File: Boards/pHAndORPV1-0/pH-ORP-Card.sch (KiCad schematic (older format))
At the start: 118 parts, among them IC1 PIC32MM0064GPM028, P1 ICSP, P2 AquaPicBus, P3 Power, P4 pH, P5 pH/ORP, Q1 NX7002AK, Q2 NX7002AK, Q3 NX7002AK, Q4 AO3407A, Q5 MMBT3904, Q6 MMBT3904, Q7 AO3407A, Q8 AO3407A, U1 AP2114H, U10 LTC2483, U11 Si8602, U12 TC7660, U2 ST485EC, U3 LMC6061, U4 TLV272, U5 LTC2483, U6 Si8602, U7 TC7660, U8 LMC6061, U9 TLV272, X1 8MHz

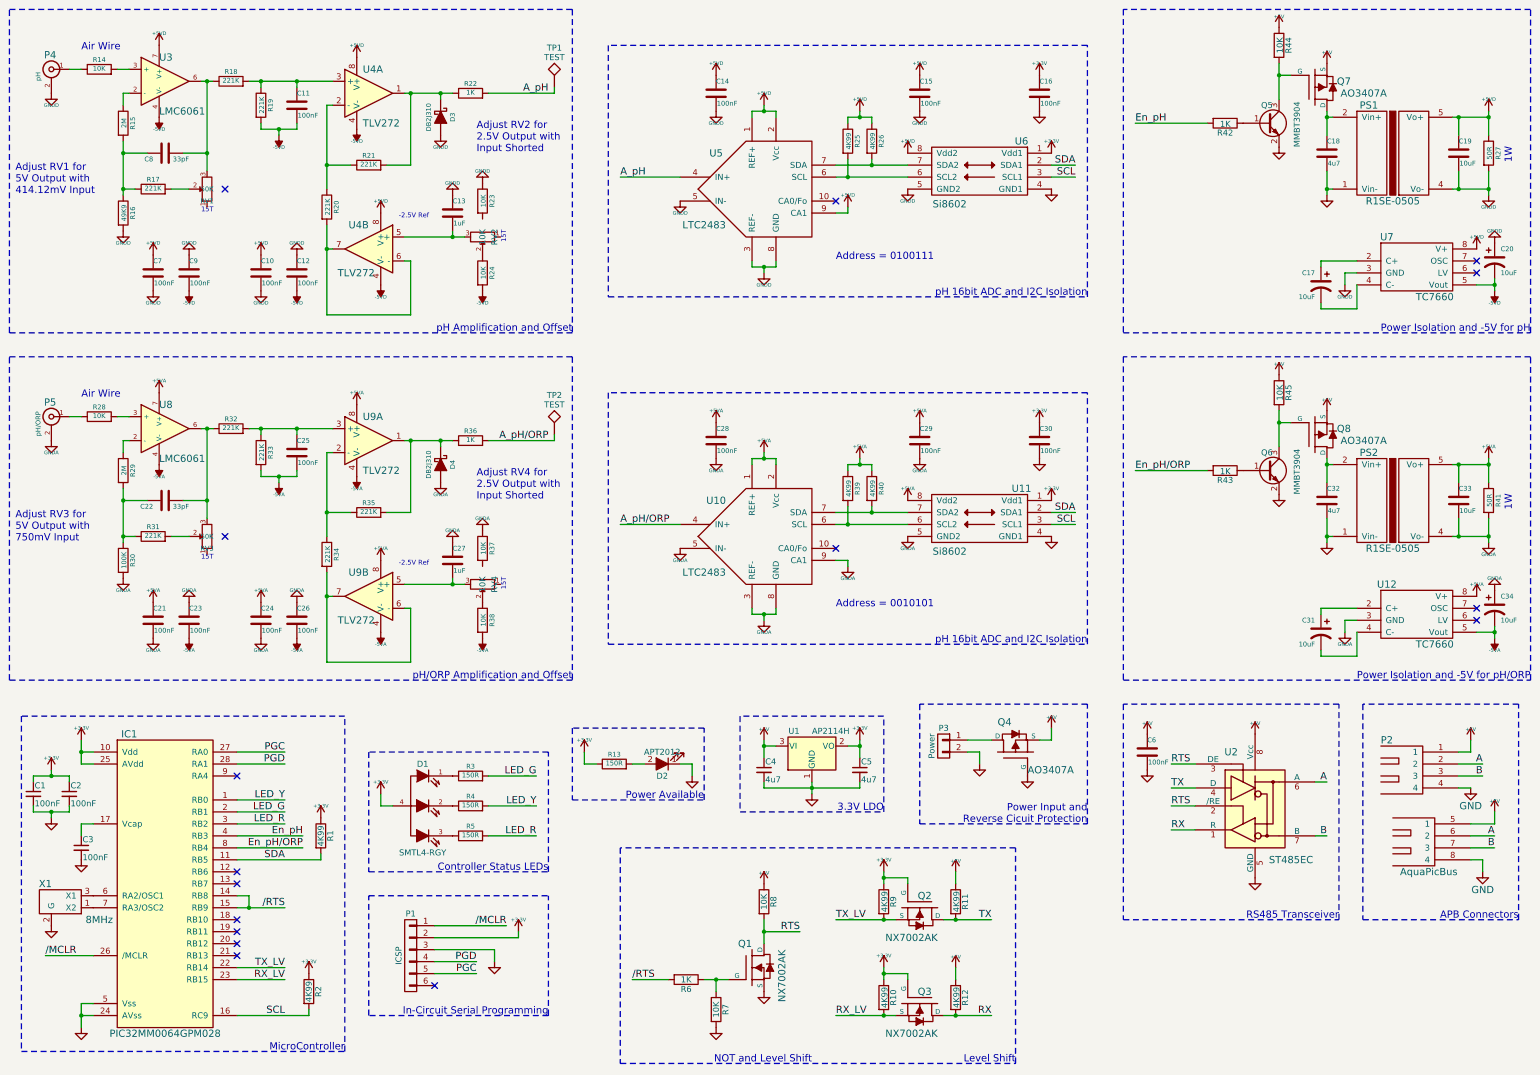
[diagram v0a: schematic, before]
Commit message: kicad updating something
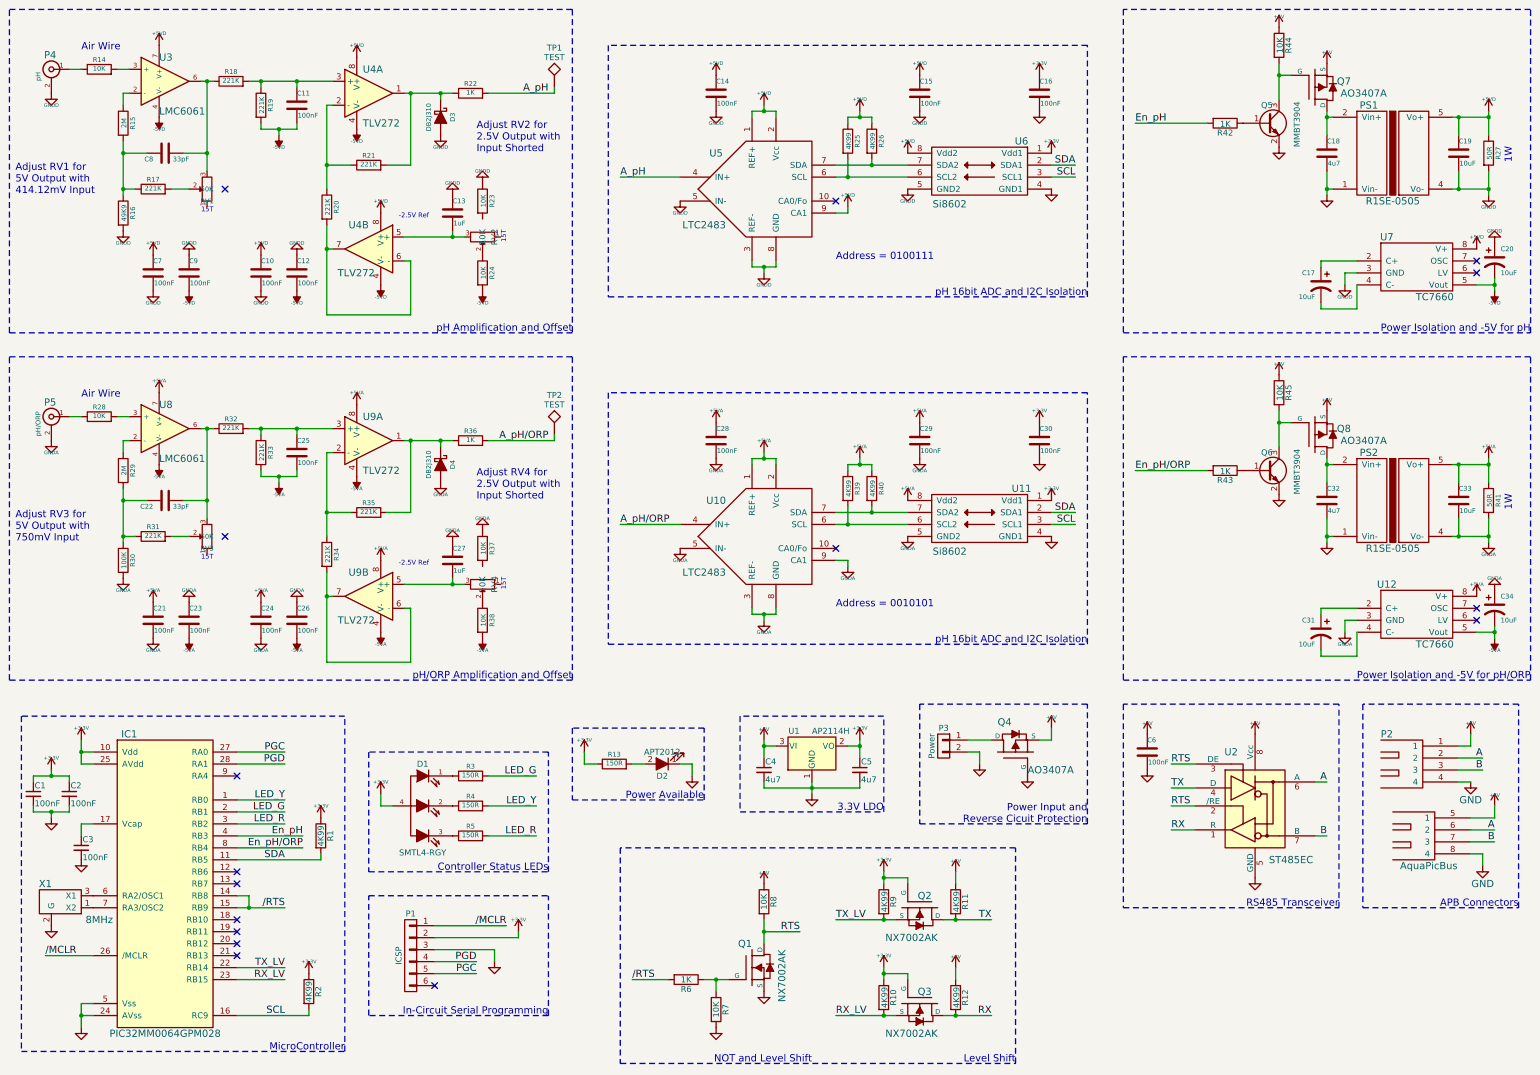
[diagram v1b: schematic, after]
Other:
- moved on the sheet: P2
